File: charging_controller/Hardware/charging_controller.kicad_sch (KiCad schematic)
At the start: 43 parts, among them J1 XT60, J10 CAN, J11 HALL1, J12 HALL2, J2 XT60, J3 ??, J4 Conn_01x08_Pin, J5 Conn_01x01, J6 Conn_01x01, J7 BAT_CONN, J8 Conn_01x01, J9 Conn_01x01, M1 Motor_DC, Q1 PMOS, Q2 NMOS, SW1 SW_Push, U1 STM32F103CBTx, U2 NCP114BSN330T1G, U3 ACS712xLCTR-20A

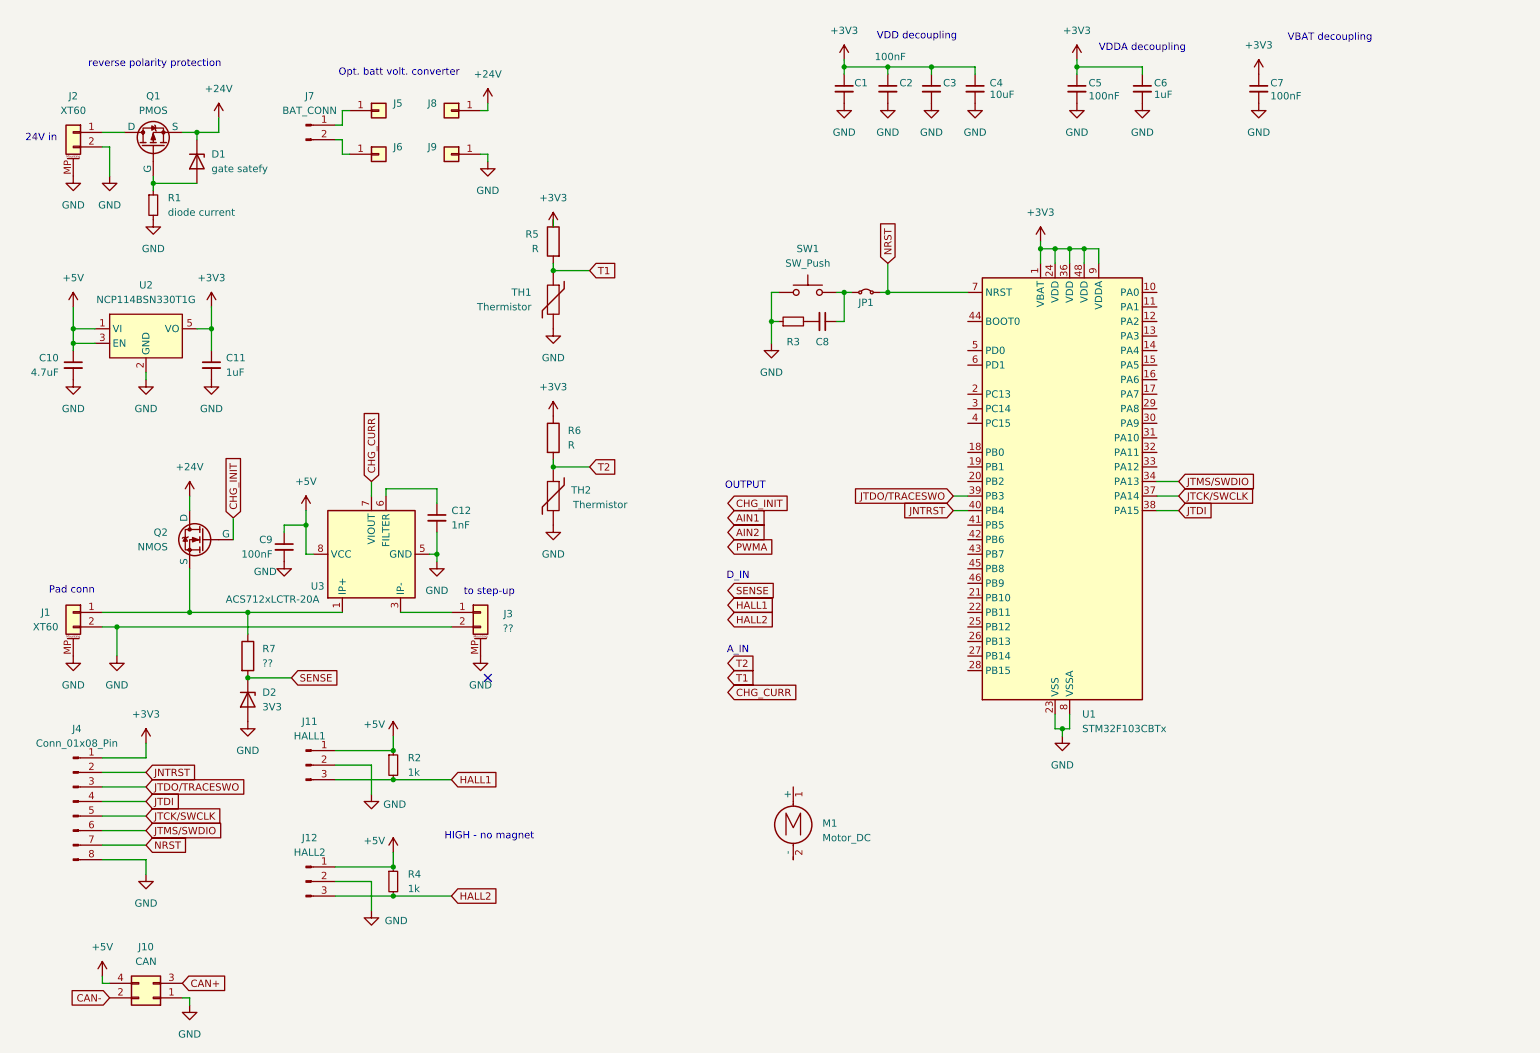
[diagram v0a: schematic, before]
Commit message: handoff_to_office
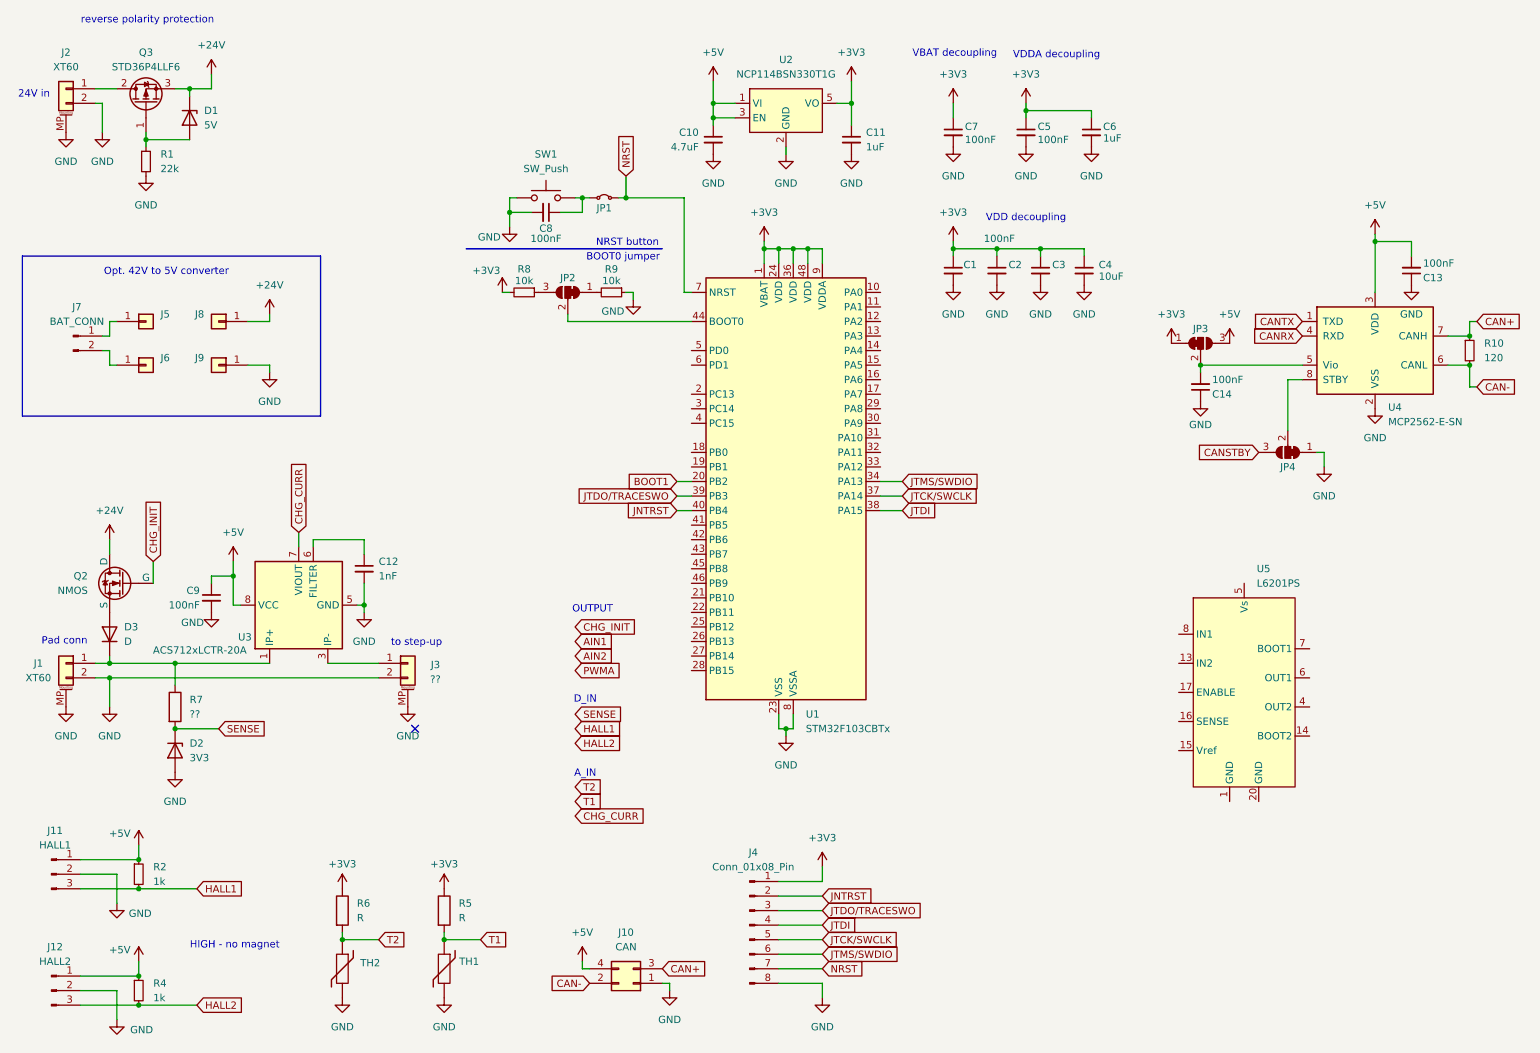
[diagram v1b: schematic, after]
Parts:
- removed M1: Motor_DC, symbol Motor:Motor_DC
- removed Q1: PMOS, symbol Simulation_SPICE:PMOS
- removed R3: R_Small, symbol Device:R_Small
- added C13, C14: 100nF, Capacitor_SMD:C_0805_2012Metric, symbol Device:C_Small
- added D3: D, symbol Device:D
- added JP2, JP3, JP4: SolderJumper_3_Bridged12, Jumper:SolderJumper-3_P1.3mm_Bridged12_RoundedPad1.0x1.5mm, symbol Jumper:SolderJumper_3_Bridged12
- added Q3: STD36P4LLF6, Package_TO_SOT_SMD:TO-252-2, symbol Device:Q_PMOS_GDS
- added R10: 120, symbol Device:R_Small
- added R8, R9: 10k, symbol Device:R_Small
- added U4: MCP2562-E-SN, Package_SO:SOIC-8_3.9x4.9mm_P1.27mm, symbol Interface_CAN_LIN:MCP2562-E-SN
- added U5: L6201PS, Package_SO:HSOP-20-1EP_11.0x15.9mm_P1.27mm_SlugDown, symbol FIRO_collected:L6201PS
- C1, C10, C11, C2, C3, C4, C5, C6, C7: footprint (none) -> Capacitor_SMD:C_0805_2012Metric
- C8: value C_Small -> 100nF; footprint (none) -> Capacitor_SMD:C_0805_2012Metric
- D1: value gate satefy -> 5V
- J1, J2: footprint (none) -> firo_footprints:AMASS_XT60PW-F-MP
- J10: footprint (none) -> Connector_TE-Connectivity:TE_Micro-MaTch_215079-4_2x02_P1.27mm_Vertical
- J4: footprint (none) -> Connector_PinHeader_2.54mm:PinHeader_2x08_P2.54mm_Vertical
- R1: value diode current -> 22k
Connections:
- net +24V: now also Q3.3 (S)
- net +3V3: now also JP3.1 (A), R8.2
- net +5V: now also C13.2, JP3.3 (B), U4.3 (VDD)
- net CAN+: now also R10.1, U4.7 (CANH)
- net CAN-: now also R10.2, U4.6 (CANL)
- net GND: now also C8.2, C13.1, C14.1, JP4.1 (A), R9.1, U4.2 (VSS)
- net at J1.1 (Pin_1), R7.1, U3.1 (IP+)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: now also D3.1 (K); no longer Q2.3 (S)
- net BOOT1: now reaches U1.20 (PB2)
- net at U1.44 (BOOT0): now also JP2.2 (C)
- net at J2.1 (Pin_1): now also Q3.2 (D)
- net at D1.2 (A), R1.1: now also Q3.1 (G)
- new net: JP2.1 (A), R9.2
- new net: JP2.3 (B), R8.1
- new net: JP4.2 (C), U4.8 (STBY)
- new net: D3.2 (A), Q2.3 (S)
- new net: C14.2, JP3.2 (C), U4.5 (Vio)
- new net: U5.1 (GND), U5.10 (GND)
- new net: U5.11 (GND), U5.20 (GND)
- new net CANRX: U4.4 (RXD)
- new net CANSTBY: JP4.3 (B)
- new net CANTX: U4.1 (TXD)
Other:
- note added: "BOOT0 jumper"
- note added: "NRST button"
- note added: "Opt. 42V to 5V converter"
- note removed: "Opt. batt volt. converter"
- moved on the sheet: C1, C10, C11, C12, C2, C3, C4, C5, C6, C7, C8, C9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
